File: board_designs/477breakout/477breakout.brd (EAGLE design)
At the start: 94.5 x 49.5 mm, 22 parts, among them IC1 PIC24FJ128GA006, J1 RJ11-6PTH, J2 5.5x2.1mm Barrel, U2 3.3V/150mA, U3 5V

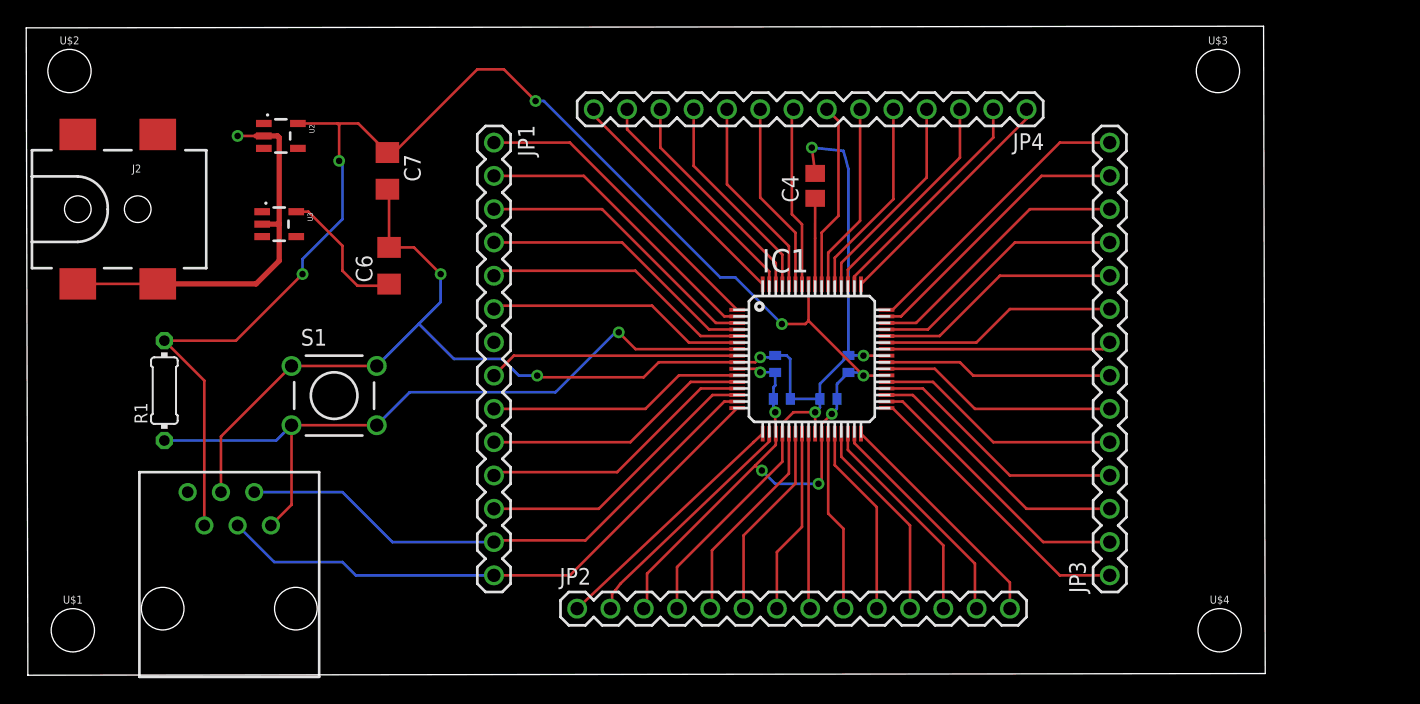
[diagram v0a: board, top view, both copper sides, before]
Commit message: Board Changes
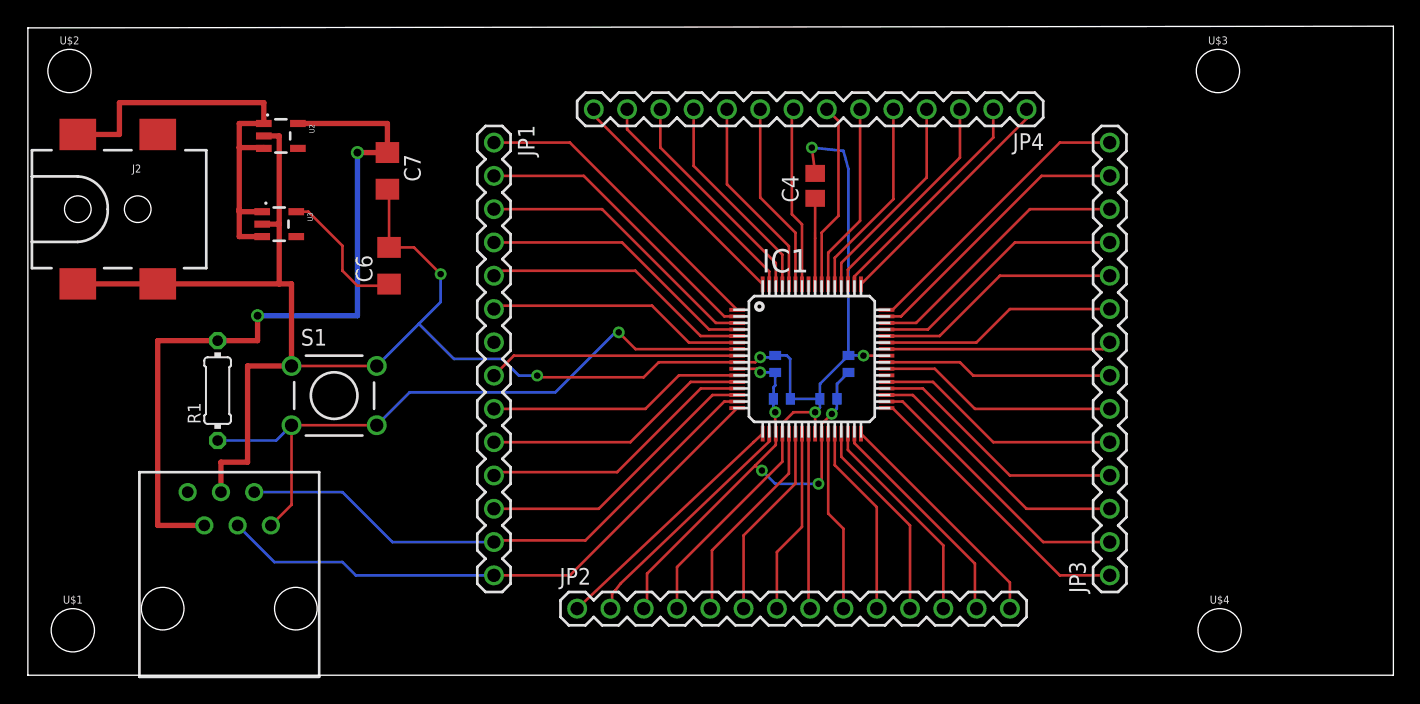
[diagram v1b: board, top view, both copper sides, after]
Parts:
- moved R1 4.06 mm to (14.5, 21.7)
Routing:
- net VCC: track 143.6 -> 98.9 mm, vias 10 -> 7
- net N$2: track 0.00 -> 34.3 mm
- net GND: track 153.7 -> 162.6 mm, vias 7 -> 6
- net MCLR: track 56.0 -> 51.9 mm
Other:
- board size 94.5 x 49.5 mm -> 104.2 x 49.5 mm
